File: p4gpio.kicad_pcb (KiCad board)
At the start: 4 copper layers, 88.9 x 22.9 mm, 92 parts, among them J1 C2760486, J10 Conn_01x04_Socket, J2 C2760486, J3 Conn_01x08_Pin, J4 Conn_01x08_Pin, J5 Conn_01x08_Pin, J6 Conn_01x08_Pin, J7 Conn_01x08_Pin, J8 Conn_01x08_Pin, J9 Conn_01x04_Socket, Q1 MBT3906DW1, Q2 AO3401A, Q3 MBT3906DW1, Q4 AO3401A, U1 TLV62569DBV, U3 W25Q128JVS, U4 TLV62569DBV, Y1 40MHz(+-10 ppm) C501798

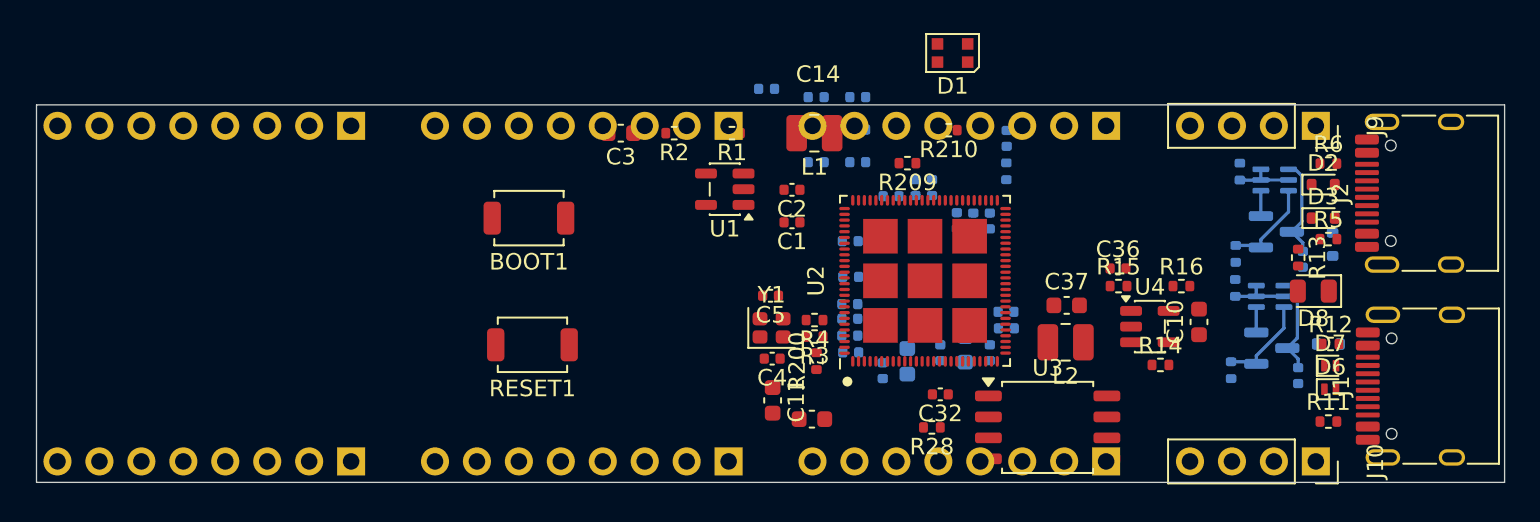
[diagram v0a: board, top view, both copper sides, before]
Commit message: Lots more routing and placement
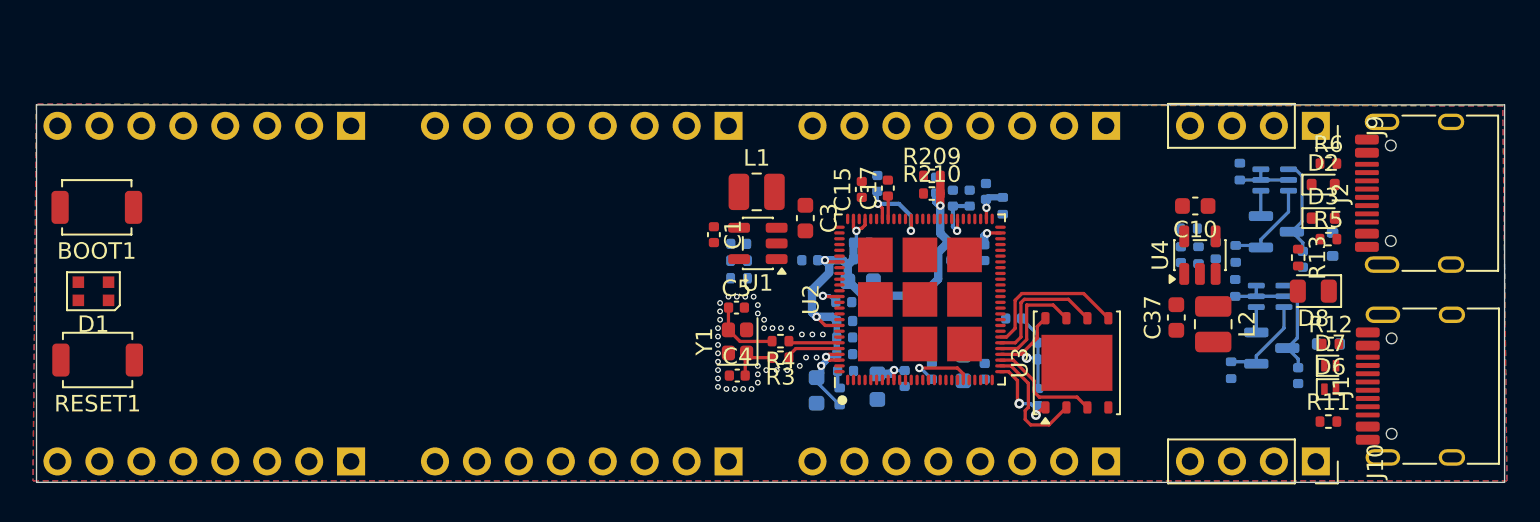
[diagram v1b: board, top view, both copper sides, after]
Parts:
- removed C19, C22: 1uF, Capacitor_SMD:C_0402_1005Metric
- C11, C14, C2, C32, C36, R1, R14, R15, R16, R2, R200, R28: moved to B.Cu
- C15, C17: moved to F.Cu
- U3: footprint Package_SO:SOIC-8_5.3x5.3mm_P1.27mm -> Package_SON:WSON-8-1EP_6x5mm_P1.27mm_EP3.4x4.3mm
- moved D1 54.0 mm to (126.1, 84.2)
- moved RESET1 26.3 mm to (126.4, 88.3)
- moved BOOT1 26.2 mm to (126.3, 79.1)
- moved C3 12.3 mm to (169.2, 79.7), turned to -90 degrees
- moved R2 9.62 mm to (165.2, 83.4)
- moved C16 9.23 mm to (172.6, 81.2)
- moved L2 9.01 mm to (193.9, 86.2), turned to -90 degrees
- moved C14 8.86 mm to (172.6, 83.6), turned to 0 degrees
- moved R1 7.73 mm to (165.2, 82.3), turned to 0 degrees
- moved R14 7.70 mm to (194.1, 81.7), turned to 90 degrees
- moved C10 7.02 mm to (192.9, 79.0), turned to 180 degrees
- moved R28 6.68 mm to (183.3, 90.6), turned to 90 degrees
- moved C37 6.68 mm to (191.7, 85.8), turned to 90 degrees
- moved C13 6.49 mm to (172.6, 82.2)
- moved C32 6.39 mm to (181.9, 85.8)
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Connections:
- C30 pad 1: /Minimal P4 V3/VDDO_FLASH -> /Minimal P4 V3/VDD_FLASH
- C31 pad 1: /Minimal P4 V3/VDDO_FLASH -> /Minimal P4 V3/VDD_FLASH
- C32 pad 1: /Minimal P4 V3/VDDO_FLASH -> /Minimal P4 V3/VDD_FLASH
- C8 pad 1: +3.3V -> /Minimal P4 V3/VDD_HP
- R28 pad 2: /Minimal P4 V3/VDDO_FLASH -> /Minimal P4 V3/VDD_FLASH
- U2 pad 1: /Minimal P4 V3/GPIO1/ADC -> /B1_1
- U2 pad 10: /Minimal P4 V3/GPIO9/ADC -> /B2_1
- U2 pad 104: /Minimal P4 V3/GPIO0/ADC -> /B1_0
- U2 pad 11: /Minimal P4 V3/GPIO10/ADC -> /B2_2
- U2 pad 12: /Minimal P4 V3/GPIO11/ADC -> /B2_3
- U2 pad 13: /Minimal P4 V3/GPIO12/ADC -> /B2_4
- U2 pad 14: /Minimal P4 V3/GPIO13/ADC -> /B2_5
- U2 pad 15: /Minimal P4 V3/GPIO14/ADC -> /B2_6
- U2 pad 16: /Minimal P4 V3/GPIO15/ADC -> /B2_7
- U2 pad 17: /Minimal P4 V3/GPIO16/ADC -> /B3_0
- U2 pad 18: /Minimal P4 V3/GPIO17/ADC -> /B3_1
- U2 pad 19: /Minimal P4 V3/GPIO18/ADC -> /B3_2
- U2 pad 2: /Minimal P4 V3/GPIO2/ADC -> /B1_2
- U2 pad 20: /Minimal P4 V3/GPIO19/ADC -> /B3_3
- U2 pad 22: /Minimal P4 V3/GPIO20/ADC -> /B3_4
- U2 pad 23: /Minimal P4 V3/GPIO21/ADC -> /B3_5
- U2 pad 24: /Minimal P4 V3/GPIO22/ADC -> /B3_6
- U2 pad 25: /Minimal P4 V3/GPIO23/ADC -> /B3_7
- U2 pad 3: /Minimal P4 V3/GPIO3/ADC -> /B1_3
- U2 pad 30: /Minimal P4 V3/VDDO_FLASH -> /Minimal P4 V3/VDD_FLASH
- U2 pad 4: /Minimal P4 V3/GPIO4/ADC -> /B1_4
- U2 pad 5: /Minimal P4 V3/GPIO5/ADC -> /B1_5
- U2 pad 6: /Minimal P4 V3/GPIO6/ADC -> /B1_6
- U2 pad 7: /Minimal P4 V3/GPIO7/ADC -> /B1_7
- U2 pad 73: /Minimal P4 V3/VDDO_3 -> unconnected-(U2-VDDO_3-Pad73)
- U2 pad 74: /Minimal P4 V3/VDDO_4 -> unconnected-(U2-VDDO_4-Pad74)
- U2 pad 8: /Minimal P4 V3/GPIO8/ADC -> /B2_0
- U2 pad 86: /Minimal P4 V3/GPIO44 -> /T1_7
- U2 pad 87: /Minimal P4 V3/GPIO45 -> /T1_6
- U2 pad 88: /Minimal P4 V3/GPIO46 -> /T1_5
- U2 pad 89: /Minimal P4 V3/GPIO47 -> /T1_4
- U2 pad 90: /Minimal P4 V3/GPIO48 -> /T1_3
- U2 pad 91: +3.3V -> /Minimal P4 V3/VDD_HP
- U2 pad 92: /Minimal P4 V3/GPIO49/ADC -> /T1_2
- U2 pad 93: /Minimal P4 V3/GPIO50/ADC -> /T1_1
- U2 pad 94: /Minimal P4 V3/GPIO51/ADC -> /T1_0
- U3 pad 8: /Minimal P4 V3/VDDO_FLASH -> /Minimal P4 V3/VDD_FLASH
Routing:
- net +3.3V: track 0.00 -> 53.6 mm, vias 0 -> 9
- net /Minimal P4 V3/VDDO_PSRAM: track 0.00 -> 11.9 mm, vias 0 -> 3
- net /Minimal P4 V3/VDD_FLASH: track 0.00 -> 9.81 mm, vias 0 -> 1
- net /Minimal P4 V3/FLASH_D: track 0.00 -> 9.24 mm
- net /Minimal P4 V3/FLASH_CK: track 0.00 -> 8.05 mm
- net /Minimal P4 V3/FLASH_Q: track 0.00 -> 7.46 mm
- net /Minimal P4 V3/FLASH_WP: track 0.00 -> 6.84 mm
- net /Minimal P4 V3/FLASH_HOLD: track 0.00 -> 6.64 mm
- net /Minimal P4 V3/FLASH_CS: track 0.00 -> 5.26 mm, vias 0 -> 2
- net Net-(C5-Pad1): track 0.00 -> 4.29 mm
- net Net-(U2-XTAL_P): track 0.00 -> 3.36 mm
- net Net-(U2-XTAL_N): track 0.00 -> 3.10 mm
- net Net-(C4-Pad2): track 0.00 -> 3.06 mm
- net Net-(U2-VDD_HP_1): track 0.00 -> 2.26 mm, vias 0 -> 1
- net /Minimal P4 V3/VDD_HP: track 0.00 -> 1.97 mm, vias 0 -> 1
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- added copper zone on B.Cu, net GND
- added copper zone on F.Cu, net GND
- added copper zone on In1.Cu, net GND
